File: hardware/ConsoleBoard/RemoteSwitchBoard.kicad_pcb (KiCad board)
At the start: 2 copper layers, 70.7 x 50 mm, 51 parts, among them J1 Conn_Coaxial, J2 Conn_01x05, J3 Conn_01x02, J4 Conn_01x02, J5 Conn_01x04, J6 Conn_01x04, J7 Conn_01x02, J8 Conn_01x05, J9 Conn_01x02, SW1 SW_Push, SW2 SW_Push, U1 STM32F303K8Tx, U2 Wio-E5, U3 3.3V, Y1 Crystal_GND2

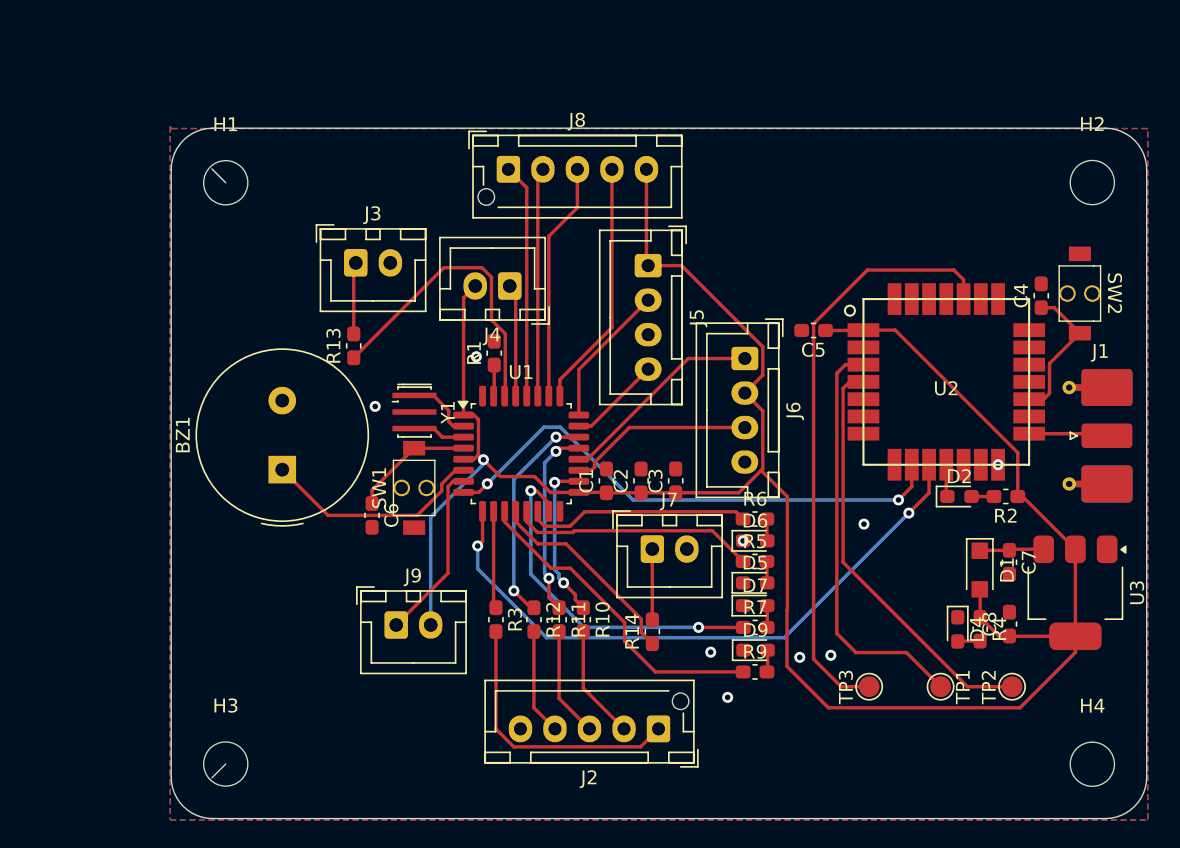
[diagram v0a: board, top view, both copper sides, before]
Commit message: update
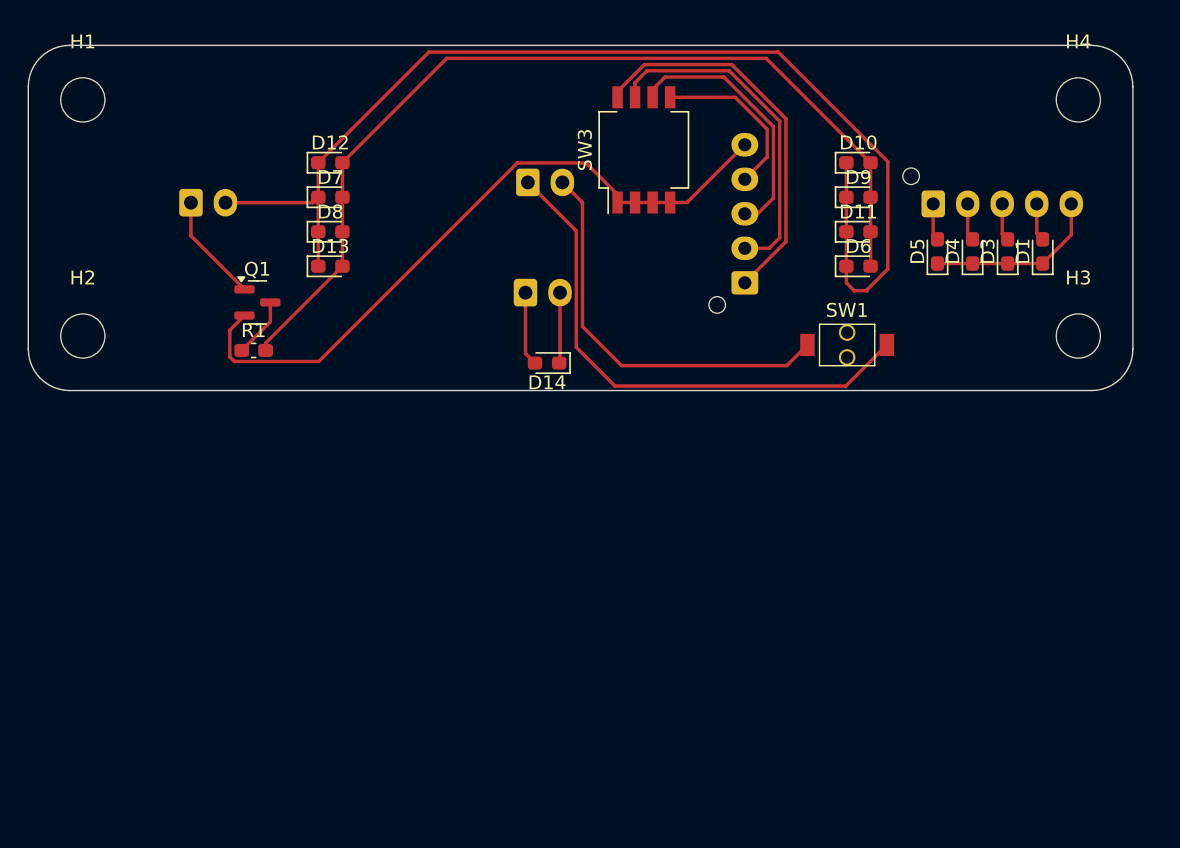
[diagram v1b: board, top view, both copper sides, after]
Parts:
- removed BZ1: Buzzer, Buzzer_Beeper:Buzzer_TDK_PS1240P02BT_D12.2mm_H6.5mm
- removed C1, C2, C4, C6: 0.1u, Capacitor_SMD:C_0603_1608Metric_Pad1.08x0.95mm_HandSolder
- removed C3, C5: 4.7u, Capacitor_SMD:C_0603_1608Metric_Pad1.08x0.95mm_HandSolder
- removed C7, C8: 10u, Capacitor_SMD:C_0603_1608Metric_Pad1.08x0.95mm_HandSolder
- removed D2: LED, LED_SMD:LED_0603_1608Metric_Pad1.05x0.95mm_HandSolder
- removed J1: Conn_Coaxial, Connector_Coaxial:SMA_Molex_73251-2120_EdgeMount_Horizontal
- removed J5, J6: Conn_01x04, Connector_JST:JST_XH_B4B-XH-A_1x04_P2.50mm_Vertical
- removed J9: Conn_01x02, Connector_JST:JST_XH_B2B-XH-A_1x02_P2.50mm_Vertical
- removed R10, R11, R12, R13, R14, R2, R3, R4, R5, R6, R7, R9: 1k, Capacitor_SMD:C_0603_1608Metric_Pad1.08x0.95mm_HandSolder
- removed SW2: SW_Push, GN10_Parts:TVAF
- removed TP1, TP2, TP3: TestPoint, TestPoint:TestPoint_Pad_D1.5mm
- removed U1: STM32F303K8Tx, Package_QFP:LQFP-32_7x7mm_P0.8mm
- removed U2: Wio-E5, GN10_Parts:LoRa-E5
- removed U3: 3.3V, Package_TO_SOT_SMD:SOT-223-3_TabPin2
- removed Y1: Crystal_GND2, Crystal:Resonator_SMD_Murata_CSTxExxV-3Pin_3.0x1.1mm_HandSoldering
- added D10: LED, LED_SMD:LED_0603_1608Metric_Pad1.05x0.95mm_HandSolder, F.Cu at (114.1, 27.5)
- added D11: LED, LED_SMD:LED_0603_1608Metric_Pad1.05x0.95mm_HandSolder, F.Cu at (114.1, 32.5)
- added D12: LED, LED_SMD:LED_0603_1608Metric_Pad1.05x0.95mm_HandSolder, F.Cu at (75.9, 27.5)
- added D13: LED, LED_SMD:LED_0603_1608Metric_Pad1.05x0.95mm_HandSolder, F.Cu at (75.9, 35.0)
- added D14: LED, LED_SMD:LED_0603_1608Metric_Pad1.05x0.95mm_HandSolder, F.Cu at (91.6, 42.0)
- added D3: LED, LED_SMD:LED_0603_1608Metric_Pad1.05x0.95mm_HandSolder, F.Cu at (124.9, 33.9)
- added D8: LED, LED_SMD:LED_0603_1608Metric_Pad1.05x0.95mm_HandSolder, F.Cu at (75.9, 32.5)
- added Q1: AO3400A, Package_TO_SOT_SMD:SOT-23, F.Cu at (70.6, 37.6)
- added SW3: SW_DIP_x04, Button_Switch_SMD:SW_DIP_SPSTx04_Slide_Copal_CHS-04B_W7.62mm_P1.27mm, F.Cu at (98.6, 26.6)
- D1: value D -> LED; footprint Diode_SMD:Nexperia_CFP3_SOD-123W -> LED_SMD:LED_0603_1608Metric_Pad1.05x0.95mm_HandSolder
- J2, J3, J4, J7, J8: moved to B.Cu
- R1: value 10k -> 1k
- moved H2 74.0 mm to (57.9, 40.1)
- moved H3 69.1 mm to (130.1, 40.1)
- moved H4 48.1 mm to (130.1, 22.9)
- moved J2 42.9 mm to (119.5, 30.5), turned to 0 degrees
- moved D7 42.7 mm to (75.9, 30.0)
- moved D9 33.6 mm to (114.1, 30.0)
- moved SW1 33.0 mm to (113.3, 40.7), turned to 0 degrees
- moved D5 27.4 mm to (119.8, 33.9), turned to 90 degrees
- moved D4 27.4 mm to (122.4, 33.9), turned to 90 degrees
- moved D1 23.5 mm to (127.5, 33.9), turned to 90 degrees
- moved D6 21.2 mm to (114.1, 35.0)
- moved J7 20.7 mm to (90.0, 36.9)
- moved J8 19.0 mm to (105.9, 36.2), turned to 90 degrees
- moved R1 17.4 mm to (70.3, 41.1), turned to 0 degrees
- moved J3 12.7 mm to (65.8, 30.4)
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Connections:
- D1 pad 1: +5V -> Net-(D1-K)
- D1 pad 2: +3.3V -> Net-(D1-A)
- D4 pad 1: GND -> Net-(D1-K)
- D5 pad 1: GND -> Net-(D1-K)
- D6 pad 1: GND -> Net-(D10-K)
- D6 pad 2: Net-(D6-A) -> Net-(D10-A)
- D7 pad 1: GND -> Net-(D10-K)
- D7 pad 2: Net-(D7-A) -> Net-(D10-A)
- D9 pad 1: GND -> Net-(D10-K)
- D9 pad 2: Net-(D9-A) -> Net-(D10-A)
- J2 pad 1: Net-(J2-Pin_1) -> Net-(D5-A)
- J2 pad 2: Net-(J2-Pin_2) -> Net-(D4-A)
- J2 pad 4: Net-(J2-Pin_4) -> Net-(D1-A)
- J2 pad 5: GND -> Net-(D1-K)
- J3 pad 2: GND -> Net-(D10-K)
- J4 pad 1: bustop -> Net-(J4-Pin_1)
- J4 pad 2: +3.3V -> Net-(J4-Pin_2)
- J7 pad 2: GND -> Net-(D14-K)
- J8 pad 1: DIP_1 -> Net-(J8-Pin_1)
- J8 pad 2: DIP_2 -> Net-(J8-Pin_2)
- J8 pad 3: DIP_3 -> Net-(J8-Pin_3)
- J8 pad 4: DIP_4 -> Net-(J8-Pin_4)
- R1 pad 2: GND -> Net-(D10-A)
- SW1 pad 1: GND -> Net-(J4-Pin_2)
- SW1 pad 2: MCU_RST -> Net-(J4-Pin_1)
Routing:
- net +3.3V: track 160.6 -> 50.1 mm, vias 1 -> 0
- net Net-(D10-K): track 0.00 -> 82.6 mm
- net Net-(D10-A): track 0.00 -> 67.9 mm
- net USART2_RX: track 45.4 -> 0.00 mm, vias 2 -> 0
- net RF_BOOT: track 43.3 -> 0.00 mm
- net USART2_TX: track 38.6 -> 0.00 mm, vias 2 -> 0
- net Net-(J4-Pin_1): track 0.00 -> 38.3 mm
- net RF_SWCLK: track 30.2 -> 0.00 mm
- net RF_SWDIO: track 30.1 -> 0.00 mm
- net Net-(J4-Pin_2): track 0.00 -> 29.1 mm
- net Net-(J8-Pin_1): track 0.00 -> 28.2 mm
- net LED_Error: track 25.3 -> 0.00 mm, vias 2 -> 0
- net Net-(J8-Pin_2): track 0.00 -> 24.7 mm
- net LED_2: track 23.3 -> 0.00 mm
- net LED_emstop: track 22.0 -> 0.00 mm
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- removed copper zone on B.Cu, net GND
- removed copper zone on F.Cu, net GND
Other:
- board size 70.7 x 50 mm -> 80 x 25 mm
